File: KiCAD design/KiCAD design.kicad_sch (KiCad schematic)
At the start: 0 parts

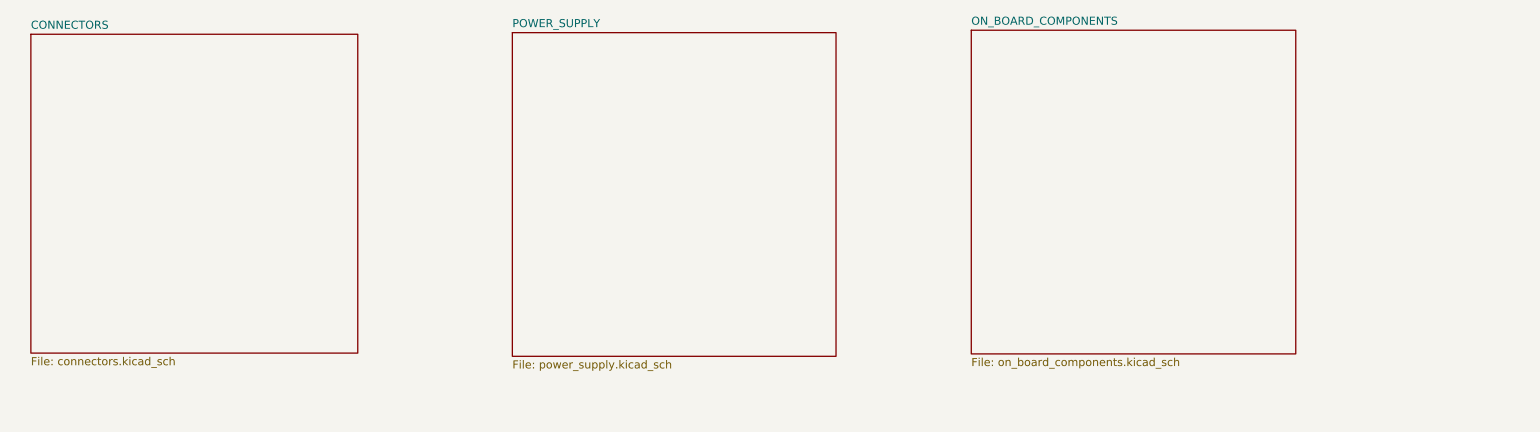
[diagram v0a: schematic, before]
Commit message: correction of errors
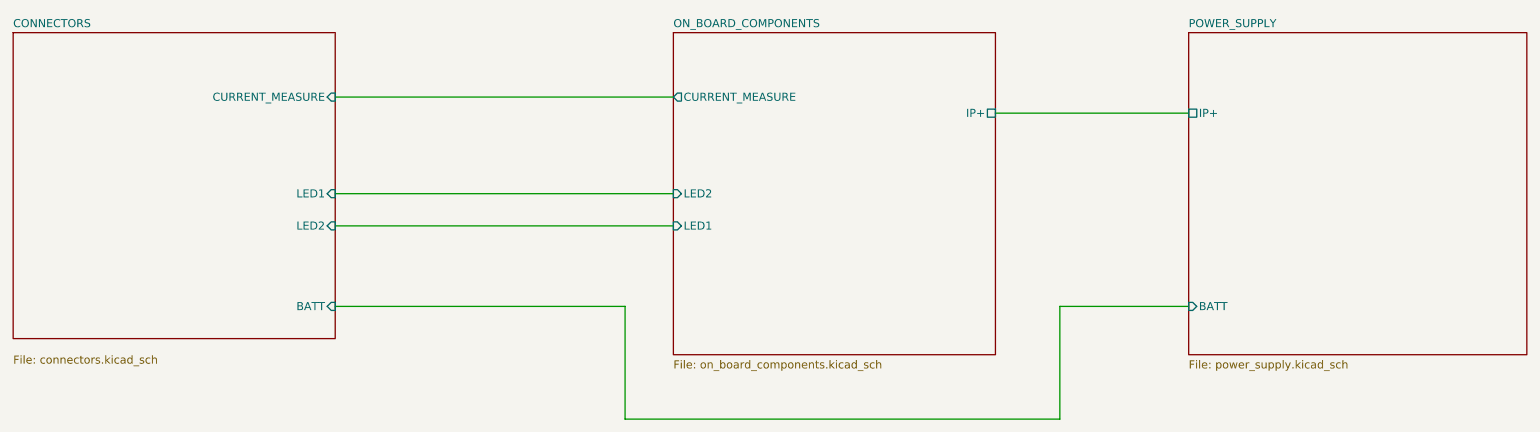
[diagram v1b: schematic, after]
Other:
- sheet CONNECTORS ports: added BATT, CURRENT_MEASURE, LED1, LED2; removed none
- sheet ON_BOARD_COMPONENTS ports: added CURRENT_MEASURE, IP+, LED1, LED2; removed none
- sheet POWER_SUPPLY ports: added BATT, IP+; removed none
